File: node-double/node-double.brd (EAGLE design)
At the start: 35.1 x 24.3 mm, 33 parts, among them IC1 TP4056, IC3 24C02, U1 ATMEGA328P_TQFP, U2 3.3V/150mA

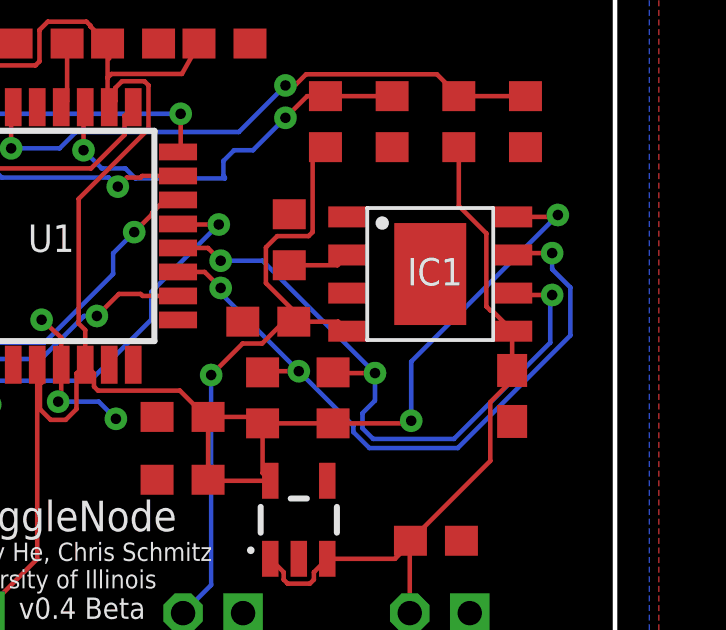
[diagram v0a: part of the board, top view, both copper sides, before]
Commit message: Node: Tweaked TP4056 activation point
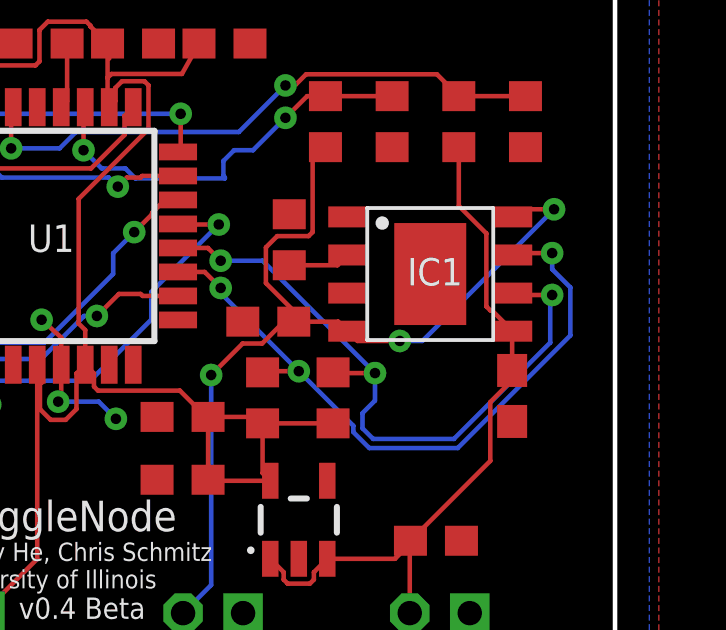
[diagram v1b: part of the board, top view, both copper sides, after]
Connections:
- net VCC: no longer IC1.8
- net VIN: now also IC1.8
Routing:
- net VCC: track 100.4 -> 87.3 mm, vias 5 -> 3
- net VIN: track 21.4 -> 31.7 mm, vias 1 -> 3
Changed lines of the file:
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@@
 <grid distance="2.5" unitdist="mil" unit="mil" style="lines" multiple="1" display="yes" altdistance="10" altunitdist="mil" altunit="mil"/>
 <layers>
-<layer number="1" name="Top" color="4" fill="1" visible="no" active="yes"/>
+<layer number="1" name="Top" color="4" fill="1" visible="yes" active="yes"/>
 <layer number="2" name="Route2" color="1" fill="3" visible="no" active="no"/>
 <layer number="3" name="Route3" color="4" fill="3" visible="no" active="no"/>
@@
 <layer number="19" name="Unrouted" color="6" fill="1" visible="yes" active="yes"/>
 <layer number="20" name="Dimension" color="24" fill="1" visible="yes" active="yes"/>
-<layer number="21" name="tPlace" color="7" fill="1" visible="no" active="yes"/>
+<layer number="21" name="tPlace" color="7" fill="1" visible="yes" active="yes"/>
 <layer number="22" name="bPlace" color="7" fill="1" visible="yes" active="yes"/>
-<layer number="23" name="tOrigins" color="15" fill="1" visible="no" active="yes"/>
+<layer number="23" name="tOrigins" color="15" fill="1" visible="yes" active="yes"/>
 <layer number="24" name="bOrigins" color="15" fill="1" visible="yes" active="yes"/>
-<layer number="25" name="tNames" color="7" fill="1" visible="no" active="yes"/>
+<layer number="25" name="tNames" color="7" fill="1" visible="yes" active="yes"/>
 <layer number="26" name="bNames" color="7" fill="1" visible="yes" active="yes"/>
-<layer number="27" name="tValues" color="7" fill="1" visible="no" active="yes"/>
-<layer number="28" name="bValues" color="7" fill="1" visible="no" active="yes"/>
+<layer number="27" name="tValues" color="7" fill="1" visible="yes" active="yes"/>
+<layer number="28" name="bValues" color="7" fill="1" visible="yes" active="yes"/>
 <layer number="29" name="tStop" color="7" fill="3" visible="no" active="yes"/>
 <layer number="30" name="bStop" color="7" fill="6" visible="no" active="yes"/>
@@
 <layer number="37" name="tTest" color="7" fill="1" visible="no" active="yes"/>
 <layer number="38" name="bTest" color="7" fill="1" visible="no" active="yes"/>
-<layer number="39" name="tKeepout" color="4" fill="11" visible="no" active="yes"/>
+<layer number="39" name="tKeepout" color="4" fill="11" visible="yes" active="yes"/>
 <layer number="40" name="bKeepout" color="1" fill="11" visible="yes" active="yes"/>
-<layer number="41" name="tRestrict" color="4" fill="10" visible="no" active="yes"/>
+<layer number="41" name="tRestrict" color="4" fill="10" visible="yes" active="yes"/>
 <layer number="42" name="bRestrict" color="1" fill="10" visible="yes" active="yes"/>
 <layer number="43" name="vRestrict" color="2" fill="10" visible="no" active="yes"/>
-<layer number="44" name="Drills" color="7" fill="1" visible="no" active="yes"/>
+<layer number="44" name="Drills" color="7" fill="1" visible="yes" active="yes"/>
 <layer number="45" name="Holes" color="7" fill="1" visible="yes" active="yes"/>
 <layer number="46" name="Milling" color="3" fill="1" visible="no" active="yes"/>
@@
 <layer number="49" name="Reference" color="7" fill="1" visible="no" active="yes"/>
 <layer number="50" name="dxf" color="7" fill="1" visible="no" active="no"/>
-<layer number="51" name="tDocu" color="7" fill="1" visible="no" active="yes"/>
+<layer number="51" name="tDocu" color="7" fill="1" visible="yes" active="yes"/>
 <layer number="52" name="bDocu" color="7" fill="1" visible="yes" active="yes"/>
 <layer number="53" name="tGND_GNDA" color="7" fill="9" visible="no" active="no"/>
@@
 <contactref element="U1" pad="6"/>
 <contactref element="R5" pad="2"/>
-<contactref element="IC1" pad="8"/>
 <contactref element="R4" pad="2"/>
 <contactref element="C7" pad="1"/>
@@
 <wire x1="39.0332" y1="41.1284875" x2="39.0332" y2="40.6908" width="0.1524" layer="1"/>
 <wire x1="39.0332" y1="40.6908" x2="38.83" y2="40.4876" width="0.1524" layer="1"/>
-<wire x1="52.28" y1="36.83" x2="53.721" y2="36.83" width="0.1524" layer="1"/>
-<wire x1="53.721" y1="36.83" x2="53.7845" y2="36.8935" width="0.1524" layer="1"/>
-<via x="53.7845" y="36.8935" extent="1-16" drill="0.35"/>
-<wire x1="53.7845" y1="36.8935" x2="48.895" y2="32.004" width="0.1524" layer="16"/>
-<wire x1="48.895" y1="32.004" x2="48.895" y2="30.0355" width="0.1524" layer="16"/>
-<via x="48.895" y="30.0355" extent="1-16" drill="0.35"/>
-<wire x1="48.895" y1="30.0355" x2="48.807" y2="29.9475" width="0.1524" layer="1"/>
-<wire x1="48.807" y1="29.9475" x2="46.2915" y2="29.9475" width="0.1524" layer="1"/>
 </signal>
 <signal name="RST">
@@
 <wire x1="42.2275" y1="31.5595" x2="42.2275" y2="24.5585" width="0.1524" layer="16"/>
 <wire x1="42.2275" y1="24.5585" x2="41.291" y2="23.622" width="0.1524" layer="16"/>
+<contactref element="IC1" pad="8"/>
+<wire x1="52.28" y1="36.83" x2="52.534" y2="37.084" width="0.1524" layer="1"/>
+<wire x1="52.534" y1="37.084" x2="53.6575" y2="37.084" width="0.1524" layer="1"/>
+<via x="53.6575" y="37.084" extent="1-16" drill="0.35"/>
+<wire x1="53.6575" y1="37.084" x2="49.2679" y2="32.6944" width="0.1524" layer="16"/>
+<wire x1="49.2679" y1="32.6944" x2="48.514" y2="32.6944" width="0.1524" layer="16"/>
+<via x="48.514" y="32.6944" extent="1-16" drill="0.35"/>
+<wire x1="48.514" y1="32.6944" x2="47.1056" y2="32.6944" width="0.1524" layer="1"/>
+<wire x1="47.1056" y1="32.6944" x2="46.78" y2="33.02" width="0.1524" layer="1"/>
 </signal>
 <signal name="PROG">
